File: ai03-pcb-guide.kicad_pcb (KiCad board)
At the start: 2 copper layers, 100 x 81 mm, 22 parts, among them U1 MOUDLE-SEEEDUINO-XIAO

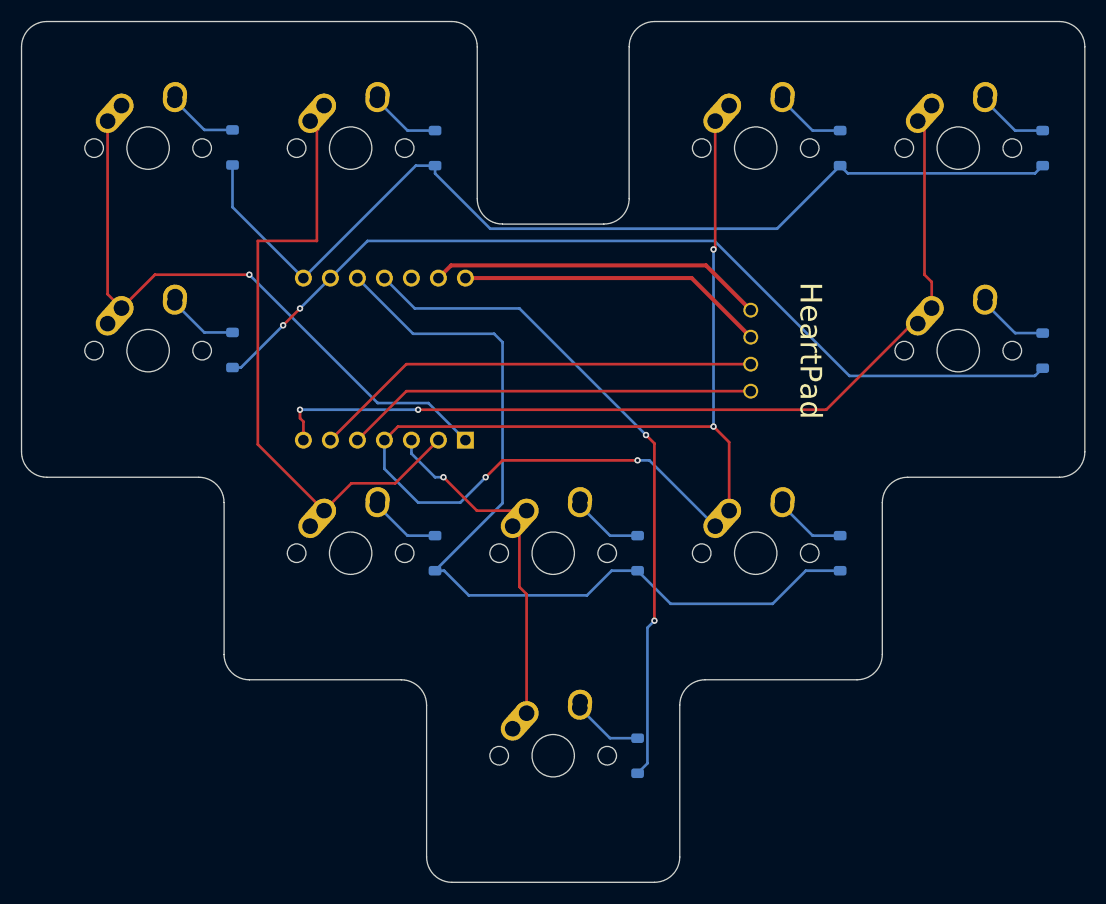
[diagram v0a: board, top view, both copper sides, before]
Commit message: a commit
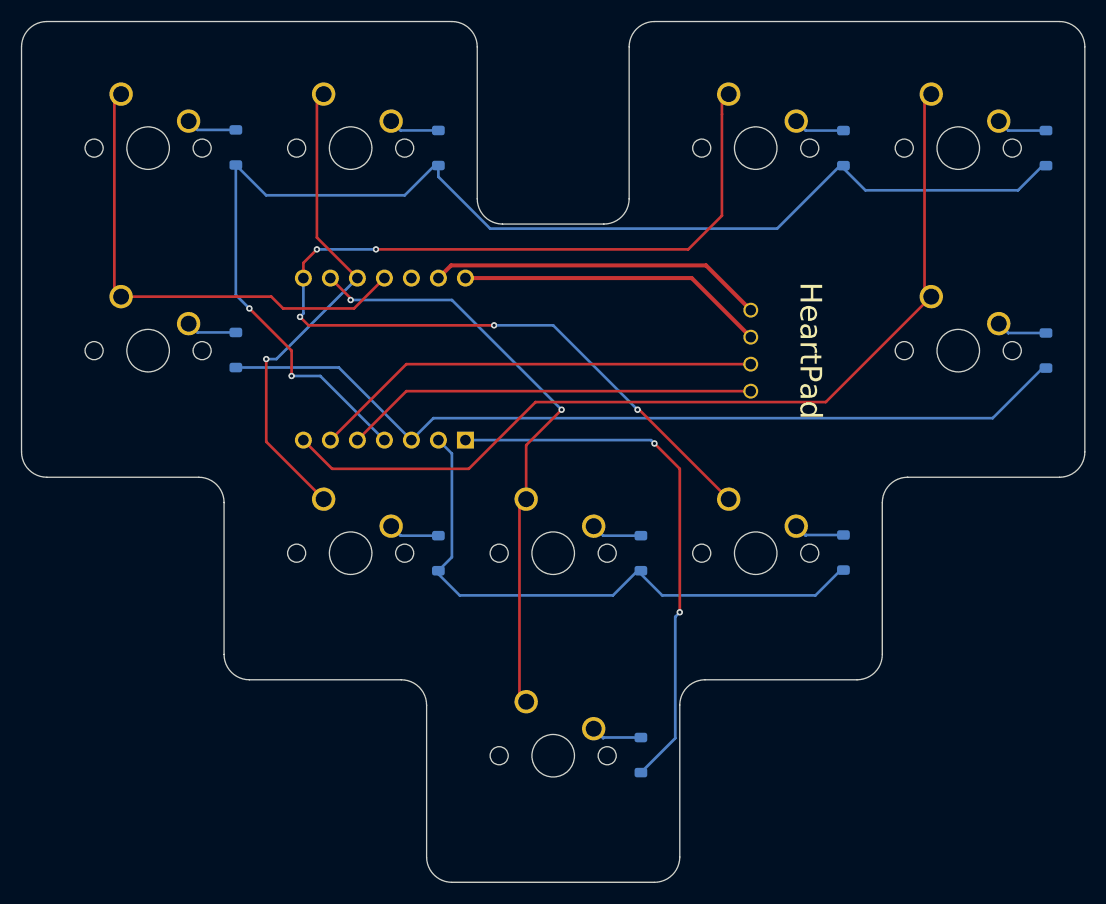
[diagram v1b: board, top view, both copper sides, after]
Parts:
- MX1, MX10, MX2, MX3, MX4, MX5, MX6, MX7, MX8, MX9: footprint MX_Alps_Hybrid:MX-1U-NoLED -> Button_Switch_Keyboard:SW_Cherry_MX_1.00u_PCB; moved to B.Cu
- moved MX3 5.68 mm to (86.4, 63.2), turned to 180 degrees
- moved MX5 5.68 mm to (143.5, 44.1), turned to 180 degrees
- moved MX9 5.68 mm to (143.5, 82.2), turned to 180 degrees
- moved MX1 5.68 mm to (86.4, 44.1), turned to 180 degrees
- moved MX10 5.68 mm to (124.5, 101.3), turned to 180 degrees
- moved MX2 5.68 mm to (105.4, 44.1), turned to 180 degrees
- moved MX4 5.68 mm to (105.4, 82.2), turned to 180 degrees
- moved MX7 5.68 mm to (162.6, 63.2), turned to 180 degrees
- moved MX8 5.68 mm to (124.5, 82.2), turned to 180 degrees
- moved MX6 5.68 mm to (162.6, 44.1), turned to 180 degrees
- moved D10 0.32 mm to (135.2, 106.3)
- moved D9 0.32 mm to (154.3, 87.2)
- moved D7 0.31 mm to (173.3, 68.2)
- moved D2 0.31 mm to (116.2, 49.2)
- moved D1 0.31 mm to (97.2, 49.1)
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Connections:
- U1 pad 1: COL 0 -> ROW 3
- U1 pad 10: ROW 2 -> COL 1
- U1 pad 11: ROW 3 -> COL 0
- U1 pad 2: COL 1 -> ROW 2
- U1 pad 3: COL 2 -> ROW 1
- U1 pad 4: COL 3 -> ROW 0
- U1 pad 8: ROW 0 -> COL 3
- U1 pad 9: ROW 1 -> COL 2
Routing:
- net ROW 2: track 82.9 -> 55.8 mm
- net ROW 0: track 93.3 -> 119.5 mm, vias 0 -> 2
- net COL 2: track 32.5 -> 56.7 mm, vias 1 -> 2
- net COL 1: track 59.6 -> 46.3 mm, vias 0 -> 1
- net COL 0: track 59.0 -> 46.0 mm, vias 1 -> 0
- net ROW 3: track 63.5 -> 51.4 mm
- net ROW 1: track 86.7 -> 81.8 mm, vias 2 -> 0
- net COL 4: track 82.6 -> 86.5 mm, vias 2 -> 0
- net COL 3: track 108.1 -> 106.2 mm, vias 4 -> 5
- net Net-(D2-A): track 6.62 -> 4.80 mm
- net Net-(D6-A): track 6.62 -> 4.81 mm
- net Net-(D5-A): track 6.62 -> 4.81 mm
- net Net-(D4-A): track 6.62 -> 4.81 mm
- net Net-(D8-A): track 6.62 -> 4.81 mm
- net Net-(D1-A): track 6.59 -> 4.78 mm
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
